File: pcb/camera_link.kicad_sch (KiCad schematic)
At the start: 16 parts, among them J1 E5J88-00LJG2-L, J2 Conn_01x09_Female, U1 AL8861

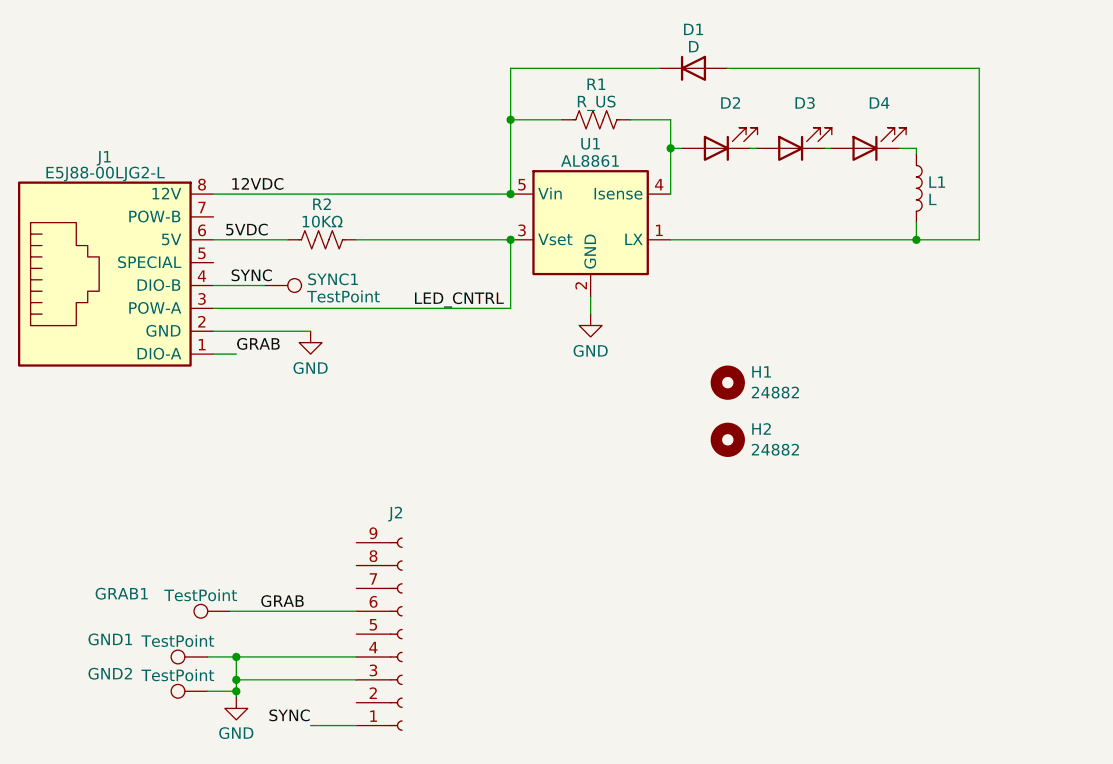
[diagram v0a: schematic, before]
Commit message: pcb v1.7
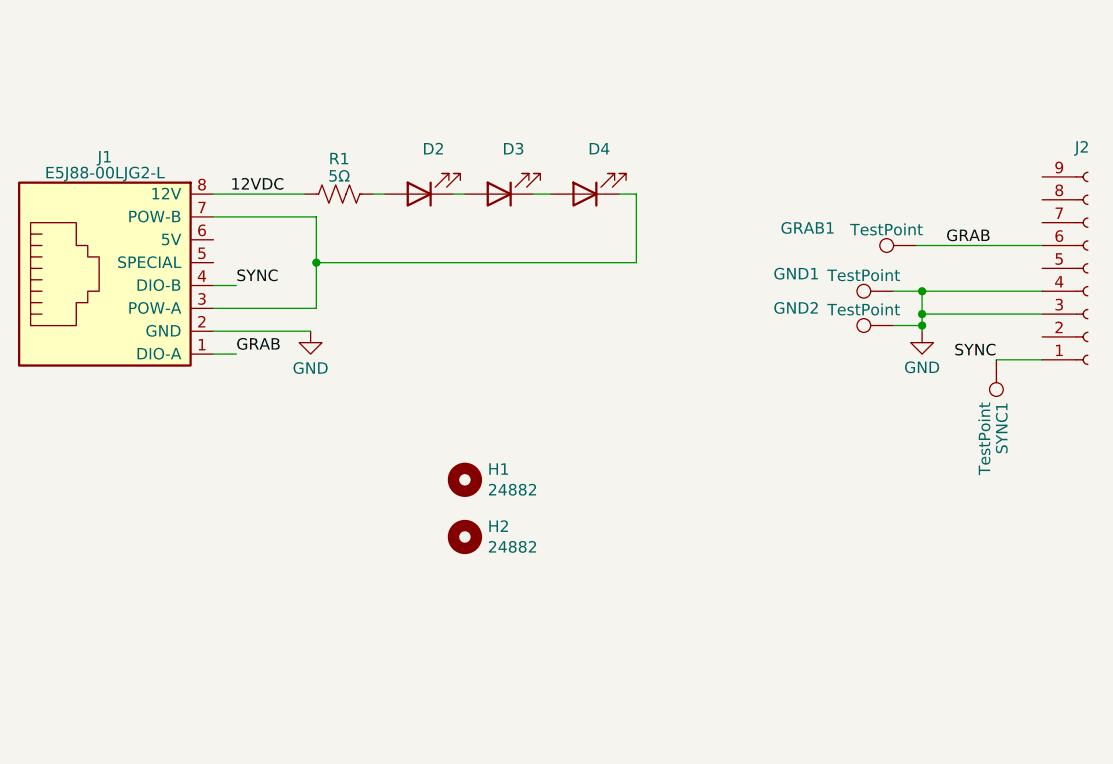
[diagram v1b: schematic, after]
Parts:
- removed D1: D, Diode_SMD:D_SMB, symbol Device:D
- removed L1: L, Inductor_THT:L_Axial_L14.5mm_D5.8mm_P7.62mm_Vertical_Fastron_HBCC, symbol Device:L
- removed R2: 10KΩ, Resistor_SMD:R_0805_2012Metric, symbol Device:R_US
- removed U1: AL8861, Package_TO_SOT_SMD:SOT-89-5, symbol asl_symbols_new:AL8861
- R1: value R_US -> 5Ω
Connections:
- net LED_CNTRL is gone; now on an unnamed net: J1.3 (POW-A)
- net at D4.1 (K): now also J1.7 (POW-B)
- net 5VDC: no longer names the net of J1.6 (5V)
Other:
- moved on the sheet: D2, D3, D4, GND1, GND2, GRAB1, H1, H2, J2, R1
